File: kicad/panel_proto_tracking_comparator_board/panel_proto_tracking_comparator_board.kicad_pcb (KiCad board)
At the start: 2 copper layers, 60 x 46.4 mm, 384 parts, among them U1 MCP6566

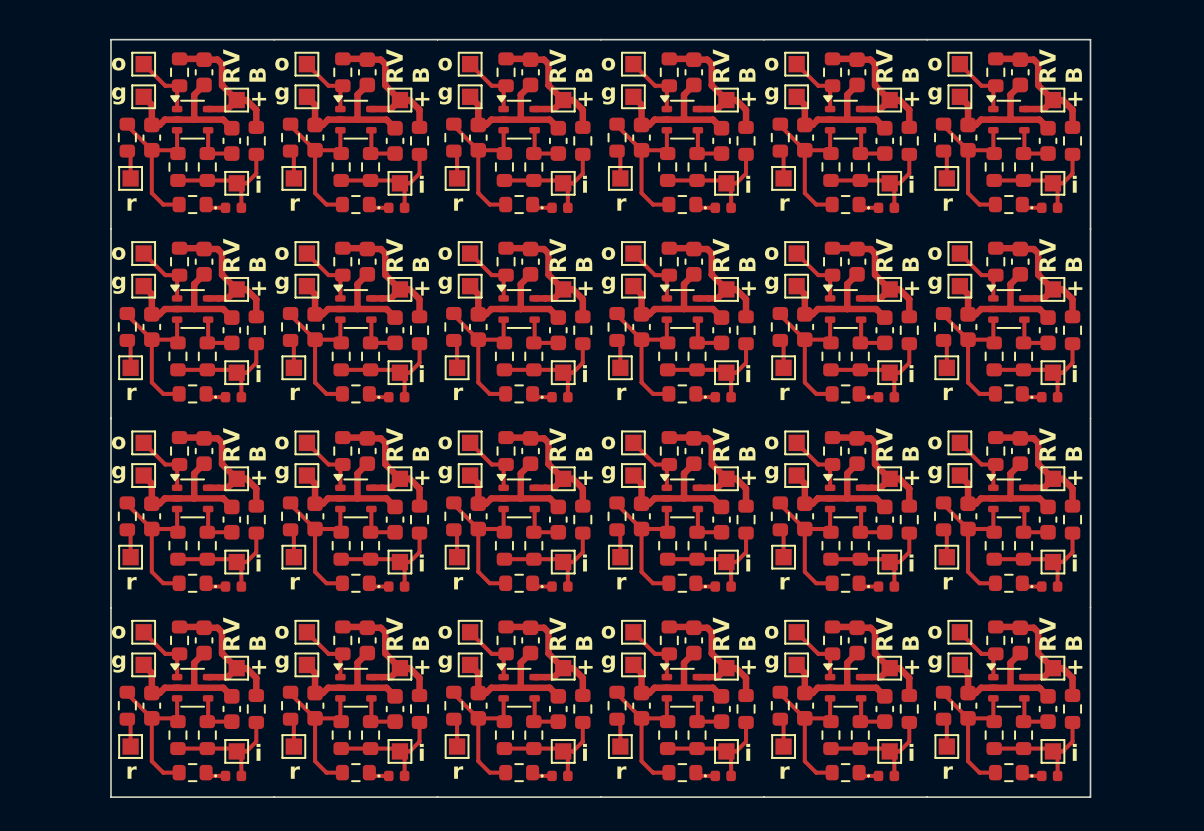
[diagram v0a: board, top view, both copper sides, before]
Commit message: Data slicer rev A
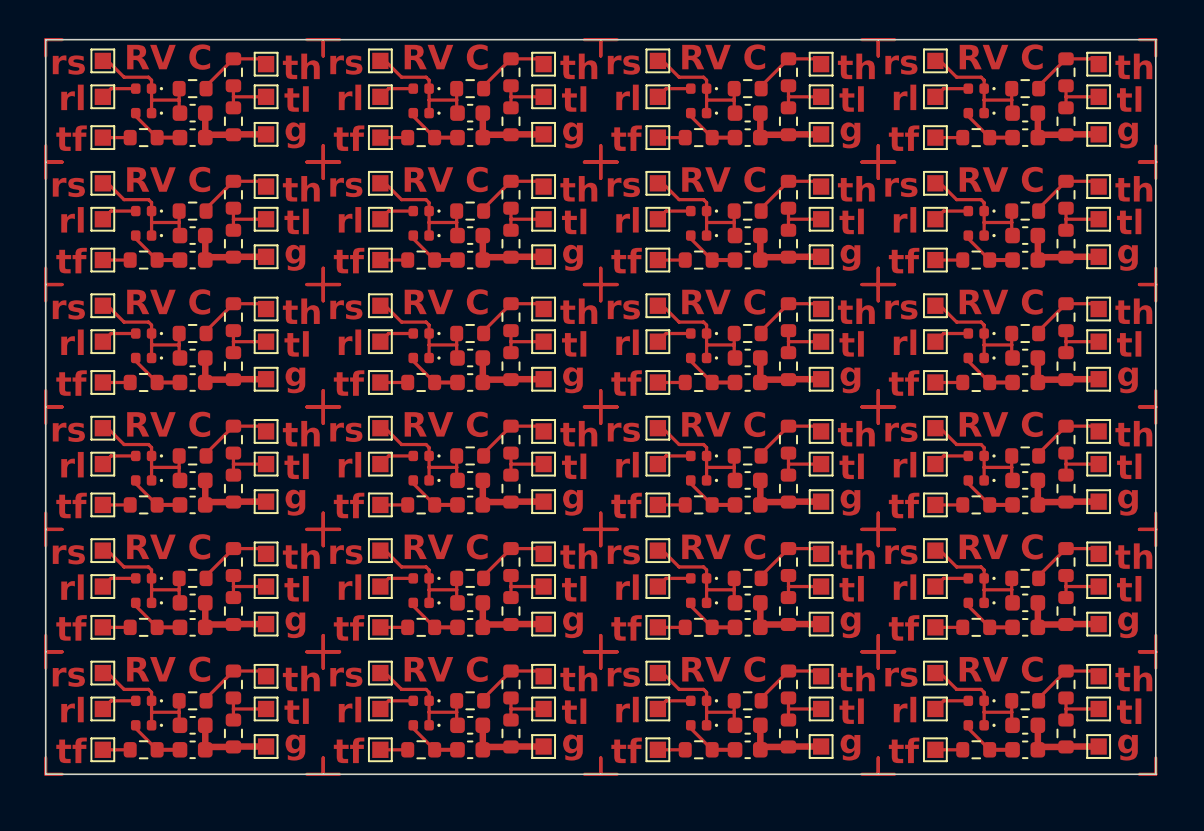
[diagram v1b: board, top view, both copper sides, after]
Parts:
- removed the C1 at (145.4, 33.6)
- removed the C1 at (125.4, 22.0)
- removed the C1 at (135.4, 33.6)
- removed the C1 at (135.4, 56.8)
- removed the C1 at (135.4, 22.0)
- removed the C1 at (135.4, 45.2)
- removed the C1 at (155.4, 33.6)
- removed the C1 at (165.4, 56.8)
- removed the C1 at (115.4, 56.8)
- removed the C1 at (115.4, 45.2)
- removed the C1 at (125.4, 56.8)
- removed the C1 at (155.4, 22.0)
- removed the C1 at (145.4, 22.0)
- removed the C1 at (145.4, 45.2)
- removed the C1 at (155.4, 45.2)
- removed the C1 at (125.4, 33.6)
- removed the C1 at (125.4, 45.2)
- removed the C1 at (165.4, 22.0)
- removed the C1 at (165.4, 33.6)
- removed the C1 at (145.4, 56.8)
- removed the C1 at (155.4, 56.8)
- removed the C1 at (115.4, 22.0)
- removed the C1 at (165.4, 45.2)
- removed the C1 at (115.4, 33.6)
- removed C2 (x24): 100pF, Capacitor_SMD:C_0603_1608Metric
- removed the C3 at (147.1, 49.4)
- removed the C3 at (127.1, 49.4)
- removed the C3 at (157.1, 61.0)
- removed the C3 at (137.1, 26.2)
- removed the C3 at (167.1, 26.2)
- removed the C3 at (157.1, 37.8)
- removed the C3 at (147.1, 61.0)
- removed the C3 at (167.1, 49.4)
- removed the C3 at (127.1, 26.2)
- removed the C3 at (167.1, 37.8)
- removed the C3 at (127.1, 61.0)
- removed the C3 at (137.1, 49.4)
- removed the C3 at (137.1, 61.0)
- removed the C3 at (147.1, 37.8)
- removed the C3 at (117.1, 61.0)
- removed the C3 at (167.1, 61.0)
- removed the C3 at (117.1, 26.2)
- removed the C3 at (127.1, 37.8)
- removed the C3 at (137.1, 37.8)
- removed the C3 at (117.1, 37.8)
- removed the C3 at (157.1, 49.4)
- removed the C3 at (157.1, 26.2)
- removed the C3 at (117.1, 49.4)
- removed the C3 at (147.1, 26.2)
- removed the D1 at (157.2, 30.3)
- removed the D1 at (137.2, 30.3)
- removed the D1 at (137.2, 53.5)
- removed the D1 at (167.2, 30.3)
- removed the D1 at (127.2, 41.9)
- removed the D1 at (127.2, 30.3)
- removed the D1 at (117.2, 41.9)
- removed the D1 at (167.2, 65.1)
- removed the D1 at (117.2, 65.1)
- removed the D1 at (167.2, 41.9)
- removed the D1 at (117.2, 30.3)
- removed the D1 at (117.2, 53.5)
- removed the D1 at (127.2, 65.1)
- removed the D1 at (157.2, 41.9)
- removed the D1 at (147.2, 65.1)
- removed the D1 at (157.2, 53.5)
- removed the D1 at (127.2, 53.5)
- removed the D1 at (157.2, 65.1)
- removed the D1 at (137.2, 65.1)
- removed the D1 at (137.2, 41.9)
- removed the D1 at (147.2, 41.9)
- removed the D1 at (147.2, 53.5)
- removed the D1 at (167.2, 53.5)
- removed the D1 at (147.2, 30.3)
- removed the R1 at (163.8, 51.0)
- removed the R1 at (143.8, 62.6)
- removed the R1 at (143.8, 51.0)
- removed the R1 at (133.8, 39.4)
- removed the R1 at (113.8, 51.0)
- removed the R1 at (133.8, 51.0)
- removed the R1 at (123.8, 51.0)
- removed the R1 at (163.8, 62.6)
- removed the R1 at (153.8, 39.4)
- removed the R1 at (113.8, 39.4)
- removed the R1 at (133.8, 27.8)
- removed the R1 at (123.8, 62.6)
- removed the R1 at (153.8, 51.0)
- removed the R1 at (123.8, 27.8)
- removed the R1 at (153.8, 62.6)
- removed the R1 at (113.8, 27.8)
- removed the R1 at (123.8, 39.4)
- removed the R1 at (143.8, 27.8)
- removed the R1 at (163.8, 27.8)
- removed the R1 at (133.8, 62.6)
- removed the R1 at (163.8, 39.4)
- removed the R1 at (143.8, 39.4)
- removed the R1 at (153.8, 27.8)
- removed the R1 at (113.8, 62.6)
- removed the R2 at (128.6, 26.2)
- removed the R2 at (118.6, 49.4)
- removed the R2 at (158.6, 37.8)
- removed the R2 at (168.6, 49.4)
- removed the R2 at (118.6, 26.2)
- removed the R2 at (118.6, 37.8)
- removed the R2 at (138.6, 61.0)
- removed the R2 at (158.6, 26.2)
- removed the R2 at (168.6, 26.2)
- removed the R2 at (148.6, 49.4)
- removed the R2 at (128.6, 37.8)
- removed the R2 at (168.6, 37.8)
- removed the R2 at (158.6, 49.4)
- removed the R2 at (128.6, 49.4)
- removed the R2 at (148.6, 61.0)
- removed the R2 at (148.6, 37.8)
- removed the R2 at (138.6, 49.4)
- removed the R2 at (128.6, 61.0)
- removed the R2 at (158.6, 61.0)
- removed the R2 at (138.6, 26.2)
- removed the R2 at (148.6, 26.2)
- removed the R2 at (168.6, 61.0)
- removed the R2 at (118.6, 61.0)
- removed the R2 at (138.6, 37.8)
- removed R3 (x24): 1k, Resistor_SMD:R_0603_1608Metric
- removed R4 (x24): 10k, Resistor_SMD:R_0603_1608Metric
- removed the R5 at (135.6, 51.0)
- removed the R5 at (145.6, 62.6)
- removed the R5 at (165.6, 39.4)
- removed the R5 at (155.6, 51.0)
- removed the R5 at (135.6, 39.4)
- removed the R5 at (115.6, 27.8)
- removed the R5 at (155.6, 27.8)
- removed the R5 at (115.6, 51.0)
- removed the R5 at (115.6, 62.6)
- removed the R5 at (115.6, 39.4)
- removed the R5 at (165.6, 51.0)
- removed the R5 at (155.6, 62.6)
- removed the R5 at (145.6, 51.0)
- removed the R5 at (125.6, 51.0)
- removed the R5 at (125.6, 62.6)
- removed the R5 at (135.6, 27.8)
- removed the R5 at (135.6, 62.6)
- removed the R5 at (145.6, 39.4)
- removed the R5 at (125.6, 27.8)
- removed the R5 at (165.6, 62.6)
- removed the R5 at (145.6, 27.8)
- removed the R5 at (165.6, 27.8)
- removed the R5 at (155.6, 39.4)
- removed the R5 at (125.6, 39.4)
- removed R6 (x24): 1M, Resistor_SMD:R_0603_1608Metric
- removed the TP1 at (157.4, 40.4)
- removed the TP1 at (117.4, 63.6)
- removed the TP1 at (137.4, 40.4)
- removed the TP1 at (117.4, 52.0)
- removed the TP1 at (167.4, 52.0)
- removed the TP1 at (147.4, 40.4)
- removed the TP1 at (127.4, 52.0)
- removed the TP1 at (167.4, 40.4)
- removed the TP1 at (147.4, 28.8)
- removed the TP1 at (127.4, 28.8)
- removed the TP1 at (117.4, 40.4)
- removed the TP1 at (127.4, 40.4)
- removed the TP1 at (147.4, 52.0)
- removed the TP1 at (137.4, 28.8)
- removed the TP1 at (117.4, 28.8)
- removed the TP1 at (157.4, 52.0)
- removed the TP1 at (167.4, 63.6)
- removed the TP1 at (167.4, 28.8)
- removed the TP1 at (137.4, 52.0)
- removed the TP1 at (157.4, 63.6)
- removed the TP1 at (157.4, 28.8)
- removed the TP1 at (127.4, 63.6)
- removed the TP1 at (147.4, 63.6)
- removed the TP1 at (137.4, 63.6)
- removed the TP2 at (151.7, 56.3)
- removed the TP2 at (151.7, 33.1)
- removed the TP2 at (121.7, 21.5)
- removed the TP2 at (111.7, 33.1)
- removed the TP2 at (141.7, 44.7)
- removed the TP2 at (131.7, 33.1)
- removed the TP2 at (151.7, 21.5)
- removed the TP2 at (161.7, 33.1)
- removed the TP2 at (141.7, 21.5)
- removed the TP2 at (141.7, 56.3)
- removed the TP2 at (121.7, 44.7)
- removed the TP2 at (151.7, 44.7)
- removed the TP2 at (141.7, 33.1)
- removed the TP2 at (161.7, 44.7)
- removed the TP2 at (131.7, 21.5)
- removed the TP2 at (121.7, 56.3)
- removed the TP2 at (111.7, 44.7)
- removed the TP2 at (121.7, 33.1)
- removed the TP2 at (131.7, 56.3)
- removed the TP2 at (111.7, 21.5)
- removed the TP2 at (161.7, 21.5)
- removed the TP2 at (111.7, 56.3)
- removed the TP2 at (131.7, 44.7)
- removed the TP2 at (161.7, 56.3)
- removed TP3 (x24): TestPoint, TestPoint:TestPoint_Pad_1.0x1.0mm
- removed the TP4 at (161.7, 46.7)
- removed the TP4 at (131.7, 58.3)
- removed the TP4 at (131.7, 46.7)
- removed the TP4 at (161.7, 23.5)
- removed the TP4 at (151.7, 46.7)
- removed the TP4 at (161.7, 35.1)
- removed the TP4 at (131.7, 23.5)
- removed the TP4 at (131.7, 35.1)
- removed the TP4 at (111.7, 58.3)
- removed the TP4 at (141.7, 46.7)
- removed the TP4 at (141.7, 35.1)
- removed the TP4 at (151.7, 58.3)
- removed the TP4 at (111.7, 35.1)
- removed the TP4 at (121.7, 58.3)
- removed the TP4 at (141.7, 58.3)
- removed the TP4 at (121.7, 35.1)
- removed the TP4 at (151.7, 35.1)
- removed the TP4 at (141.7, 23.5)
- removed the TP4 at (161.7, 58.3)
- removed the TP4 at (111.7, 46.7)
- removed the TP4 at (121.7, 23.5)
- removed the TP4 at (151.7, 23.5)
- removed the TP4 at (111.7, 23.5)
- removed the TP4 at (121.7, 46.7)
- removed the TP5 at (140.9, 28.5)
- removed the TP5 at (150.9, 51.7)
- removed the TP5 at (160.9, 40.1)
- removed the TP5 at (120.9, 40.1)
- removed the TP5 at (120.9, 28.5)
- removed the TP5 at (130.9, 63.3)
- removed the TP5 at (140.9, 40.1)
- removed the TP5 at (110.9, 63.3)
- removed the TP5 at (130.9, 51.7)
- removed the TP5 at (110.9, 40.1)
- removed the TP5 at (130.9, 28.5)
- removed the TP5 at (110.9, 51.7)
- removed the TP5 at (140.9, 51.7)
- removed the TP5 at (160.9, 63.3)
- removed the TP5 at (120.9, 51.7)
- removed the TP5 at (160.9, 28.5)
- removed the TP5 at (150.9, 28.5)
- removed the TP5 at (140.9, 63.3)
- removed the TP5 at (120.9, 63.3)
- removed the TP5 at (130.9, 40.1)
- removed the TP5 at (150.9, 63.3)
- removed the TP5 at (160.9, 51.7)
- removed the TP5 at (110.9, 28.5)
- removed the TP5 at (150.9, 40.1)
- removed U1 (x24): MCP6566, Package_TO_SOT_SMD:SOT-353_SC-70-5
- added C1: 0.1uF, Capacitor_SMD:C_0603_1608Metric, F.Cu at (165.7, 41.0)
- added C1: 0.1uF, Capacitor_SMD:C_0603_1608Metric, F.Cu at (114.7, 33.5)
- added C1: 0.1uF, Capacitor_SMD:C_0603_1608Metric, F.Cu at (165.7, 56.0)
- added C1: 0.1uF, Capacitor_SMD:C_0603_1608Metric, F.Cu at (114.7, 41.0)
- added C1: 0.1uF, Capacitor_SMD:C_0603_1608Metric, F.Cu at (114.7, 63.5)
- added C1: 0.1uF, Capacitor_SMD:C_0603_1608Metric, F.Cu at (148.7, 33.5)
- added C1: 0.1uF, Capacitor_SMD:C_0603_1608Metric, F.Cu at (114.7, 56.0)
- added C1: 0.1uF, Capacitor_SMD:C_0603_1608Metric, F.Cu at (131.7, 41.0)
- added C1: 0.1uF, Capacitor_SMD:C_0603_1608Metric, F.Cu at (114.7, 48.5)
- added C1: 0.1uF, Capacitor_SMD:C_0603_1608Metric, F.Cu at (165.7, 26.0)
- added C1: 0.1uF, Capacitor_SMD:C_0603_1608Metric, F.Cu at (165.7, 48.5)
- added C1: 0.1uF, Capacitor_SMD:C_0603_1608Metric, F.Cu at (131.7, 48.5)
- added C1: 0.1uF, Capacitor_SMD:C_0603_1608Metric, F.Cu at (131.7, 33.5)
- added C1: 0.1uF, Capacitor_SMD:C_0603_1608Metric, F.Cu at (148.7, 63.5)
- added C1: 0.1uF, Capacitor_SMD:C_0603_1608Metric, F.Cu at (165.7, 33.5)
- added C1: 0.1uF, Capacitor_SMD:C_0603_1608Metric, F.Cu at (131.7, 63.5)
- added C1: 0.1uF, Capacitor_SMD:C_0603_1608Metric, F.Cu at (131.7, 56.0)
- added C1: 0.1uF, Capacitor_SMD:C_0603_1608Metric, F.Cu at (148.7, 48.5)
- added C1: 0.1uF, Capacitor_SMD:C_0603_1608Metric, F.Cu at (114.7, 26.0)
- added C1: 0.1uF, Capacitor_SMD:C_0603_1608Metric, F.Cu at (148.7, 26.0)
- added C1: 0.1uF, Capacitor_SMD:C_0603_1608Metric, F.Cu at (131.7, 26.0)
- added C1: 0.1uF, Capacitor_SMD:C_0603_1608Metric, F.Cu at (148.7, 56.0)
- added C1: 0.1uF, Capacitor_SMD:C_0603_1608Metric, F.Cu at (165.7, 63.5)
- added C1: 0.1uF, Capacitor_SMD:C_0603_1608Metric, F.Cu at (148.7, 41.0)
- added C3: 1nF, Capacitor_SMD:C_0603_1608Metric, F.Cu at (114.7, 32.0)
- added C3: 1nF, Capacitor_SMD:C_0603_1608Metric, F.Cu at (131.7, 47.0)
- added C3: 1nF, Capacitor_SMD:C_0603_1608Metric, F.Cu at (165.7, 32.0)
- added C3: 1nF, Capacitor_SMD:C_0603_1608Metric, F.Cu at (131.7, 32.0)
- added C3: 1nF, Capacitor_SMD:C_0603_1608Metric, F.Cu at (114.7, 47.0)
- added C3: 1nF, Capacitor_SMD:C_0603_1608Metric, F.Cu at (165.7, 62.0)
- added C3: 1nF, Capacitor_SMD:C_0603_1608Metric, F.Cu at (131.7, 24.5)
- added C3: 1nF, Capacitor_SMD:C_0603_1608Metric, F.Cu at (148.7, 47.0)
- added C3: 1nF, Capacitor_SMD:C_0603_1608Metric, F.Cu at (165.7, 39.5)
- added C3: 1nF, Capacitor_SMD:C_0603_1608Metric, F.Cu at (131.7, 62.0)
- added C3: 1nF, Capacitor_SMD:C_0603_1608Metric, F.Cu at (114.7, 54.5)
- added C3: 1nF, Capacitor_SMD:C_0603_1608Metric, F.Cu at (148.7, 54.5)
- added C3: 1nF, Capacitor_SMD:C_0603_1608Metric, F.Cu at (131.7, 54.5)
- added C3: 1nF, Capacitor_SMD:C_0603_1608Metric, F.Cu at (165.7, 24.5)
- added C3: 1nF, Capacitor_SMD:C_0603_1608Metric, F.Cu at (148.7, 62.0)
- added C3: 1nF, Capacitor_SMD:C_0603_1608Metric, F.Cu at (148.7, 39.5)
- added C3: 1nF, Capacitor_SMD:C_0603_1608Metric, F.Cu at (114.7, 62.0)
- added C3: 1nF, Capacitor_SMD:C_0603_1608Metric, F.Cu at (165.7, 47.0)
- added C3: 1nF, Capacitor_SMD:C_0603_1608Metric, F.Cu at (114.7, 39.5)
- added C3: 1nF, Capacitor_SMD:C_0603_1608Metric, F.Cu at (131.7, 39.5)
- added C3: 1nF, Capacitor_SMD:C_0603_1608Metric, F.Cu at (165.7, 54.5)
- added C3: 1nF, Capacitor_SMD:C_0603_1608Metric, F.Cu at (148.7, 24.5)
- added C3: 1nF, Capacitor_SMD:C_0603_1608Metric, F.Cu at (114.7, 24.5)
- added C3: 1nF, Capacitor_SMD:C_0603_1608Metric, F.Cu at (148.7, 32.0)
- added D1: D_Schottky, Custom_Diode:D_0402_1005Metric, F.Cu at (162.7, 53.0)
- added D1: D_Schottky, Custom_Diode:D_0402_1005Metric, F.Cu at (162.7, 60.5)
- added D1: D_Schottky, Custom_Diode:D_0402_1005Metric, F.Cu at (128.7, 30.5)
- added D1: D_Schottky, Custom_Diode:D_0402_1005Metric, F.Cu at (128.7, 23.0)
- added D1: D_Schottky, Custom_Diode:D_0402_1005Metric, F.Cu at (111.7, 60.5)
- added D1: D_Schottky, Custom_Diode:D_0402_1005Metric, F.Cu at (111.7, 30.5)
- added D1: D_Schottky, Custom_Diode:D_0402_1005Metric, F.Cu at (111.7, 38.0)
- added D1: D_Schottky, Custom_Diode:D_0402_1005Metric, F.Cu at (145.7, 23.0)
- added D1: D_Schottky, Custom_Diode:D_0402_1005Metric, F.Cu at (145.7, 30.5)
- added D1: D_Schottky, Custom_Diode:D_0402_1005Metric, F.Cu at (145.7, 38.0)
- added D1: D_Schottky, Custom_Diode:D_0402_1005Metric, F.Cu at (145.7, 45.5)
- added D1: D_Schottky, Custom_Diode:D_0402_1005Metric, F.Cu at (128.7, 38.0)
- added D1: D_Schottky, Custom_Diode:D_0402_1005Metric, F.Cu at (128.7, 60.5)
- added D1: D_Schottky, Custom_Diode:D_0402_1005Metric, F.Cu at (162.7, 30.5)
- added D1: D_Schottky, Custom_Diode:D_0402_1005Metric, F.Cu at (128.7, 53.0)
- added D1: D_Schottky, Custom_Diode:D_0402_1005Metric, F.Cu at (162.7, 45.5)
- added D1: D_Schottky, Custom_Diode:D_0402_1005Metric, F.Cu at (111.7, 23.0)
- added D1: D_Schottky, Custom_Diode:D_0402_1005Metric, F.Cu at (111.7, 45.5)
- added D1: D_Schottky, Custom_Diode:D_0402_1005Metric, F.Cu at (162.7, 38.0)
- added D1: D_Schottky, Custom_Diode:D_0402_1005Metric, F.Cu at (162.7, 23.0)
- added D1: D_Schottky, Custom_Diode:D_0402_1005Metric, F.Cu at (128.7, 45.5)
- added D1: D_Schottky, Custom_Diode:D_0402_1005Metric, F.Cu at (145.7, 60.5)
- added D1: D_Schottky, Custom_Diode:D_0402_1005Metric, F.Cu at (111.7, 53.0)
- added D1: D_Schottky, Custom_Diode:D_0402_1005Metric, F.Cu at (145.7, 53.0)
- added D2: D_Schottky, Custom_Diode:D_0402_1005Metric, F.Cu at (111.7, 54.5)
- added D2: D_Schottky, Custom_Diode:D_0402_1005Metric, F.Cu at (162.7, 54.5)
- added D2: D_Schottky, Custom_Diode:D_0402_1005Metric, F.Cu at (162.7, 24.5)
- added D2: D_Schottky, Custom_Diode:D_0402_1005Metric, F.Cu at (111.7, 24.5)
- added D2: D_Schottky, Custom_Diode:D_0402_1005Metric, F.Cu at (111.7, 47.0)
- added D2: D_Schottky, Custom_Diode:D_0402_1005Metric, F.Cu at (162.7, 62.0)
- added D2: D_Schottky, Custom_Diode:D_0402_1005Metric, F.Cu at (145.7, 39.5)
- added D2: D_Schottky, Custom_Diode:D_0402_1005Metric, F.Cu at (128.7, 24.5)
- added D2: D_Schottky, Custom_Diode:D_0402_1005Metric, F.Cu at (111.7, 62.0)
- added D2: D_Schottky, Custom_Diode:D_0402_1005Metric, F.Cu at (145.7, 24.5)
- added D2: D_Schottky, Custom_Diode:D_0402_1005Metric, F.Cu at (128.7, 54.5)
- added D2: D_Schottky, Custom_Diode:D_0402_1005Metric, F.Cu at (145.7, 32.0)
- added D2: D_Schottky, Custom_Diode:D_0402_1005Metric, F.Cu at (128.7, 62.0)
- added D2: D_Schottky, Custom_Diode:D_0402_1005Metric, F.Cu at (145.7, 54.5)
- added D2: D_Schottky, Custom_Diode:D_0402_1005Metric, F.Cu at (128.7, 39.5)
- added D2: D_Schottky, Custom_Diode:D_0402_1005Metric, F.Cu at (111.7, 32.0)
- added D2: D_Schottky, Custom_Diode:D_0402_1005Metric, F.Cu at (162.7, 39.5)
- added D2: D_Schottky, Custom_Diode:D_0402_1005Metric, F.Cu at (162.7, 47.0)
- added D2: D_Schottky, Custom_Diode:D_0402_1005Metric, F.Cu at (162.7, 32.0)
- added D2: D_Schottky, Custom_Diode:D_0402_1005Metric, F.Cu at (145.7, 62.0)
- added D2: D_Schottky, Custom_Diode:D_0402_1005Metric, F.Cu at (128.7, 32.0)
- added D2: D_Schottky, Custom_Diode:D_0402_1005Metric, F.Cu at (111.7, 39.5)
- added D2: D_Schottky, Custom_Diode:D_0402_1005Metric, F.Cu at (128.7, 47.0)
- added D2: D_Schottky, Custom_Diode:D_0402_1005Metric, F.Cu at (145.7, 47.0)
- added R1: 10k, Resistor_SMD:R_0603_1608Metric, F.Cu at (111.7, 48.5)
- added R1: 10k, Resistor_SMD:R_0603_1608Metric, F.Cu at (111.7, 56.0)
- added R1: 10k, Resistor_SMD:R_0603_1608Metric, F.Cu at (145.7, 26.0)
- added R1: 10k, Resistor_SMD:R_0603_1608Metric, F.Cu at (162.7, 48.5)
- added R1: 10k, Resistor_SMD:R_0603_1608Metric, F.Cu at (162.7, 56.0)
- added R1: 10k, Resistor_SMD:R_0603_1608Metric, F.Cu at (145.7, 33.5)
- added R1: 10k, Resistor_SMD:R_0603_1608Metric, F.Cu at (162.7, 63.5)
- added R1: 10k, Resistor_SMD:R_0603_1608Metric, F.Cu at (128.7, 26.0)
- added R1: 10k, Resistor_SMD:R_0603_1608Metric, F.Cu at (111.7, 63.5)
- added R1: 10k, Resistor_SMD:R_0603_1608Metric, F.Cu at (162.7, 26.0)
- added R1: 10k, Resistor_SMD:R_0603_1608Metric, F.Cu at (145.7, 63.5)
- added R1: 10k, Resistor_SMD:R_0603_1608Metric, F.Cu at (145.7, 56.0)
- added R1: 10k, Resistor_SMD:R_0603_1608Metric, F.Cu at (162.7, 33.5)
- added R1: 10k, Resistor_SMD:R_0603_1608Metric, F.Cu at (128.7, 33.5)
- added R1: 10k, Resistor_SMD:R_0603_1608Metric, F.Cu at (145.7, 48.5)
- added R1: 10k, Resistor_SMD:R_0603_1608Metric, F.Cu at (111.7, 33.5)
- added R1: 10k, Resistor_SMD:R_0603_1608Metric, F.Cu at (128.7, 41.0)
- added R1: 10k, Resistor_SMD:R_0603_1608Metric, F.Cu at (111.7, 26.0)
- added R1: 10k, Resistor_SMD:R_0603_1608Metric, F.Cu at (128.7, 48.5)
- added R1: 10k, Resistor_SMD:R_0603_1608Metric, F.Cu at (128.7, 56.0)
- added R1: 10k, Resistor_SMD:R_0603_1608Metric, F.Cu at (162.7, 41.0)
- added R1: 10k, Resistor_SMD:R_0603_1608Metric, F.Cu at (128.7, 63.5)
- added R1: 10k, Resistor_SMD:R_0603_1608Metric, F.Cu at (145.7, 41.0)
- added R1: 10k, Resistor_SMD:R_0603_1608Metric, F.Cu at (111.7, 41.0)
- added R2: 100k, Resistor_SMD:R_0603_1608Metric, F.Cu at (134.2, 29.5)
- added R2: 100k, Resistor_SMD:R_0603_1608Metric, F.Cu at (117.2, 29.5)
- added R2: 100k, Resistor_SMD:R_0603_1608Metric, F.Cu at (168.2, 52.0)
- added R2: 100k, Resistor_SMD:R_0603_1608Metric, F.Cu at (134.2, 37.0)
- added R2: 100k, Resistor_SMD:R_0603_1608Metric, F.Cu at (151.2, 59.5)
- added R2: 100k, Resistor_SMD:R_0603_1608Metric, F.Cu at (134.2, 59.5)
- added R2: 100k, Resistor_SMD:R_0603_1608Metric, F.Cu at (168.2, 37.0)
- added R2: 100k, Resistor_SMD:R_0603_1608Metric, F.Cu at (134.2, 44.5)
- added R2: 100k, Resistor_SMD:R_0603_1608Metric, F.Cu at (151.2, 29.5)
- added R2: 100k, Resistor_SMD:R_0603_1608Metric, F.Cu at (151.2, 44.5)
- added R2: 100k, Resistor_SMD:R_0603_1608Metric, F.Cu at (134.2, 22.0)
- added R2: 100k, Resistor_SMD:R_0603_1608Metric, F.Cu at (168.2, 22.0)
- added R2: 100k, Resistor_SMD:R_0603_1608Metric, F.Cu at (117.2, 52.0)
- added R2: 100k, Resistor_SMD:R_0603_1608Metric, F.Cu at (117.2, 59.5)
- added R2: 100k, Resistor_SMD:R_0603_1608Metric, F.Cu at (151.2, 22.0)
- added R2: 100k, Resistor_SMD:R_0603_1608Metric, F.Cu at (117.2, 44.5)
- added R2: 100k, Resistor_SMD:R_0603_1608Metric, F.Cu at (168.2, 44.5)
- added R2: 100k, Resistor_SMD:R_0603_1608Metric, F.Cu at (151.2, 52.0)
- added R2: 100k, Resistor_SMD:R_0603_1608Metric, F.Cu at (117.2, 37.0)
- added R2: 100k, Resistor_SMD:R_0603_1608Metric, F.Cu at (168.2, 59.5)
- added R2: 100k, Resistor_SMD:R_0603_1608Metric, F.Cu at (117.2, 22.0)
- added R2: 100k, Resistor_SMD:R_0603_1608Metric, F.Cu at (151.2, 37.0)
- added R2: 100k, Resistor_SMD:R_0603_1608Metric, F.Cu at (168.2, 29.5)
- added R2: 100k, Resistor_SMD:R_0603_1608Metric, F.Cu at (134.2, 52.0)
- added R5: 100k, Resistor_SMD:R_0603_1608Metric, F.Cu at (165.7, 45.5)
- added R5: 100k, Resistor_SMD:R_0603_1608Metric, F.Cu at (114.7, 23.0)
- added R5: 100k, Resistor_SMD:R_0603_1608Metric, F.Cu at (131.7, 23.0)
- added R5: 100k, Resistor_SMD:R_0603_1608Metric, F.Cu at (148.7, 23.0)
- added R5: 100k, Resistor_SMD:R_0603_1608Metric, F.Cu at (131.7, 30.5)
- added R5: 100k, Resistor_SMD:R_0603_1608Metric, F.Cu at (114.7, 30.5)
- added R5: 100k, Resistor_SMD:R_0603_1608Metric, F.Cu at (165.7, 23.0)
- added R5: 100k, Resistor_SMD:R_0603_1608Metric, F.Cu at (131.7, 60.5)
- added R5: 100k, Resistor_SMD:R_0603_1608Metric, F.Cu at (148.7, 30.5)
- added R5: 100k, Resistor_SMD:R_0603_1608Metric, F.Cu at (131.7, 53.0)
- added R5: 100k, Resistor_SMD:R_0603_1608Metric, F.Cu at (165.7, 60.5)
- added R5: 100k, Resistor_SMD:R_0603_1608Metric, F.Cu at (148.7, 53.0)
- added R5: 100k, Resistor_SMD:R_0603_1608Metric, F.Cu at (131.7, 45.5)
- added R5: 100k, Resistor_SMD:R_0603_1608Metric, F.Cu at (131.7, 38.0)
- added R5: 100k, Resistor_SMD:R_0603_1608Metric, F.Cu at (148.7, 60.5)
- added R5: 100k, Resistor_SMD:R_0603_1608Metric, F.Cu at (165.7, 38.0)
- added R5: 100k, Resistor_SMD:R_0603_1608Metric, F.Cu at (148.7, 38.0)
- added R5: 100k, Resistor_SMD:R_0603_1608Metric, F.Cu at (165.7, 30.5)
- added R5: 100k, Resistor_SMD:R_0603_1608Metric, F.Cu at (114.7, 53.0)
- added R5: 100k, Resistor_SMD:R_0603_1608Metric, F.Cu at (114.7, 38.0)
- added R5: 100k, Resistor_SMD:R_0603_1608Metric, F.Cu at (148.7, 45.5)
- added R5: 100k, Resistor_SMD:R_0603_1608Metric, F.Cu at (114.7, 45.5)
- added R5: 100k, Resistor_SMD:R_0603_1608Metric, F.Cu at (114.7, 60.5)
- added R5: 100k, Resistor_SMD:R_0603_1608Metric, F.Cu at (165.7, 53.0)
- added R7: 200k, Resistor_SMD:R_0603_1608Metric, F.Cu at (134.2, 32.5)
- added R7: 200k, Resistor_SMD:R_0603_1608Metric, F.Cu at (117.2, 25.0)
- added R7: 200k, Resistor_SMD:R_0603_1608Metric, F.Cu at (117.2, 32.5)
- added R7: 200k, Resistor_SMD:R_0603_1608Metric, F.Cu at (151.2, 47.5)
- added R7: 200k, Resistor_SMD:R_0603_1608Metric, F.Cu at (117.2, 62.5)
- added R7: 200k, Resistor_SMD:R_0603_1608Metric, F.Cu at (168.2, 55.0)
- added R7: 200k, Resistor_SMD:R_0603_1608Metric, F.Cu at (168.2, 25.0)
- added R7: 200k, Resistor_SMD:R_0603_1608Metric, F.Cu at (151.2, 32.5)
- added R7: 200k, Resistor_SMD:R_0603_1608Metric, F.Cu at (134.2, 40.0)
- added R7: 200k, Resistor_SMD:R_0603_1608Metric, F.Cu at (117.2, 40.0)
- added R7: 200k, Resistor_SMD:R_0603_1608Metric, F.Cu at (151.2, 62.5)
- added R7: 200k, Resistor_SMD:R_0603_1608Metric, F.Cu at (168.2, 32.5)
- added R7: 200k, Resistor_SMD:R_0603_1608Metric, F.Cu at (134.2, 25.0)
- added R7: 200k, Resistor_SMD:R_0603_1608Metric, F.Cu at (134.2, 62.5)
- added R7: 200k, Resistor_SMD:R_0603_1608Metric, F.Cu at (168.2, 62.5)
- added R7: 200k, Resistor_SMD:R_0603_1608Metric, F.Cu at (168.2, 40.0)
- added R7: 200k, Resistor_SMD:R_0603_1608Metric, F.Cu at (134.2, 55.0)
- added R7: 200k, Resistor_SMD:R_0603_1608Metric, F.Cu at (151.2, 55.0)
- added R7: 200k, Resistor_SMD:R_0603_1608Metric, F.Cu at (151.2, 25.0)
- added R7: 200k, Resistor_SMD:R_0603_1608Metric, F.Cu at (134.2, 47.5)
- added R7: 200k, Resistor_SMD:R_0603_1608Metric, F.Cu at (151.2, 40.0)
- added R7: 200k, Resistor_SMD:R_0603_1608Metric, F.Cu at (117.2, 55.0)
- added R7: 200k, Resistor_SMD:R_0603_1608Metric, F.Cu at (168.2, 47.5)
- added R7: 200k, Resistor_SMD:R_0603_1608Metric, F.Cu at (117.2, 47.5)
- added TP1: TestPoint, TestPoint:TestPoint_Pad_1.0x1.0mm, F.Cu at (109.2, 31.0)
- added TP1: TestPoint, TestPoint:TestPoint_Pad_1.0x1.0mm, F.Cu at (126.2, 38.5)
- added TP1: TestPoint, TestPoint:TestPoint_Pad_1.0x1.0mm, F.Cu at (143.2, 46.0)
- added TP1: TestPoint, TestPoint:TestPoint_Pad_1.0x1.0mm, F.Cu at (143.2, 23.5)
- added TP1: TestPoint, TestPoint:TestPoint_Pad_1.0x1.0mm, F.Cu at (160.2, 61.0)
- added TP1: TestPoint, TestPoint:TestPoint_Pad_1.0x1.0mm, F.Cu at (143.2, 31.0)
- added TP1: TestPoint, TestPoint:TestPoint_Pad_1.0x1.0mm, F.Cu at (160.2, 31.0)
- added TP1: TestPoint, TestPoint:TestPoint_Pad_1.0x1.0mm, F.Cu at (109.2, 38.5)
- added TP1: TestPoint, TestPoint:TestPoint_Pad_1.0x1.0mm, F.Cu at (109.2, 53.5)
- added TP1: TestPoint, TestPoint:TestPoint_Pad_1.0x1.0mm, F.Cu at (126.2, 46.0)
- added TP1: TestPoint, TestPoint:TestPoint_Pad_1.0x1.0mm, F.Cu at (160.2, 53.5)
- added TP1: TestPoint, TestPoint:TestPoint_Pad_1.0x1.0mm, F.Cu at (126.2, 53.5)
- added TP1: TestPoint, TestPoint:TestPoint_Pad_1.0x1.0mm, F.Cu at (126.2, 31.0)
- added TP1: TestPoint, TestPoint:TestPoint_Pad_1.0x1.0mm, F.Cu at (160.2, 38.5)
- added TP1: TestPoint, TestPoint:TestPoint_Pad_1.0x1.0mm, F.Cu at (160.2, 23.5)
- added TP1: TestPoint, TestPoint:TestPoint_Pad_1.0x1.0mm, F.Cu at (126.2, 23.5)
- added TP1: TestPoint, TestPoint:TestPoint_Pad_1.0x1.0mm, F.Cu at (109.2, 23.5)
- added TP1: TestPoint, TestPoint:TestPoint_Pad_1.0x1.0mm, F.Cu at (143.2, 38.5)
- added TP1: TestPoint, TestPoint:TestPoint_Pad_1.0x1.0mm, F.Cu at (160.2, 46.0)
- added TP1: TestPoint, TestPoint:TestPoint_Pad_1.0x1.0mm, F.Cu at (143.2, 61.0)
- added TP1: TestPoint, TestPoint:TestPoint_Pad_1.0x1.0mm, F.Cu at (109.2, 46.0)
- added TP1: TestPoint, TestPoint:TestPoint_Pad_1.0x1.0mm, F.Cu at (109.2, 61.0)
- added TP1: TestPoint, TestPoint:TestPoint_Pad_1.0x1.0mm, F.Cu at (143.2, 53.5)
- added TP1: TestPoint, TestPoint:TestPoint_Pad_1.0x1.0mm, F.Cu at (126.2, 61.0)
- added TP2: TestPoint, TestPoint:TestPoint_Pad_1.0x1.0mm, F.Cu at (109.2, 41.0)
- added TP2: TestPoint, TestPoint:TestPoint_Pad_1.0x1.0mm, F.Cu at (126.2, 26.0)
- added TP2: TestPoint, TestPoint:TestPoint_Pad_1.0x1.0mm, F.Cu at (160.2, 41.0)
- added TP2: TestPoint, TestPoint:TestPoint_Pad_1.0x1.0mm, F.Cu at (143.2, 63.5)
- added TP2: TestPoint, TestPoint:TestPoint_Pad_1.0x1.0mm, F.Cu at (109.2, 33.5)
- added TP2: TestPoint, TestPoint:TestPoint_Pad_1.0x1.0mm, F.Cu at (160.2, 33.5)
- added TP2: TestPoint, TestPoint:TestPoint_Pad_1.0x1.0mm, F.Cu at (160.2, 48.5)
- added TP2: TestPoint, TestPoint:TestPoint_Pad_1.0x1.0mm, F.Cu at (109.2, 63.5)
- added TP2: TestPoint, TestPoint:TestPoint_Pad_1.0x1.0mm, F.Cu at (160.2, 56.0)
- added TP2: TestPoint, TestPoint:TestPoint_Pad_1.0x1.0mm, F.Cu at (160.2, 26.0)
- added TP2: TestPoint, TestPoint:TestPoint_Pad_1.0x1.0mm, F.Cu at (143.2, 56.0)
- added TP2: TestPoint, TestPoint:TestPoint_Pad_1.0x1.0mm, F.Cu at (126.2, 56.0)
- added TP2: TestPoint, TestPoint:TestPoint_Pad_1.0x1.0mm, F.Cu at (143.2, 26.0)
- added TP2: TestPoint, TestPoint:TestPoint_Pad_1.0x1.0mm, F.Cu at (143.2, 33.5)
- added TP2: TestPoint, TestPoint:TestPoint_Pad_1.0x1.0mm, F.Cu at (143.2, 48.5)
- added TP2: TestPoint, TestPoint:TestPoint_Pad_1.0x1.0mm, F.Cu at (143.2, 41.0)
- added TP2: TestPoint, TestPoint:TestPoint_Pad_1.0x1.0mm, F.Cu at (160.2, 63.5)
- added TP2: TestPoint, TestPoint:TestPoint_Pad_1.0x1.0mm, F.Cu at (126.2, 48.5)
- added TP2: TestPoint, TestPoint:TestPoint_Pad_1.0x1.0mm, F.Cu at (126.2, 63.5)
- added TP2: TestPoint, TestPoint:TestPoint_Pad_1.0x1.0mm, F.Cu at (126.2, 41.0)
- added TP2: TestPoint, TestPoint:TestPoint_Pad_1.0x1.0mm, F.Cu at (109.2, 48.5)
- added TP2: TestPoint, TestPoint:TestPoint_Pad_1.0x1.0mm, F.Cu at (109.2, 56.0)
- added TP2: TestPoint, TestPoint:TestPoint_Pad_1.0x1.0mm, F.Cu at (126.2, 33.5)
- added TP2: TestPoint, TestPoint:TestPoint_Pad_1.0x1.0mm, F.Cu at (109.2, 26.0)
- added TP4: TestPoint, TestPoint:TestPoint_Pad_1.0x1.0mm, F.Cu at (153.2, 55.8)
- added TP4: TestPoint, TestPoint:TestPoint_Pad_1.0x1.0mm, F.Cu at (119.2, 25.8)
- added TP4: TestPoint, TestPoint:TestPoint_Pad_1.0x1.0mm, F.Cu at (153.2, 25.8)
- added TP4: TestPoint, TestPoint:TestPoint_Pad_1.0x1.0mm, F.Cu at (119.2, 33.3)
- added TP4: TestPoint, TestPoint:TestPoint_Pad_1.0x1.0mm, F.Cu at (136.2, 25.8)
- added TP4: TestPoint, TestPoint:TestPoint_Pad_1.0x1.0mm, F.Cu at (136.2, 63.3)
- added TP4: TestPoint, TestPoint:TestPoint_Pad_1.0x1.0mm, F.Cu at (153.2, 40.8)
- added TP4: TestPoint, TestPoint:TestPoint_Pad_1.0x1.0mm, F.Cu at (170.2, 25.8)
- added TP4: TestPoint, TestPoint:TestPoint_Pad_1.0x1.0mm, F.Cu at (170.2, 48.3)
- added TP4: TestPoint, TestPoint:TestPoint_Pad_1.0x1.0mm, F.Cu at (170.2, 63.3)
- added TP4: TestPoint, TestPoint:TestPoint_Pad_1.0x1.0mm, F.Cu at (119.2, 48.3)
- added TP4: TestPoint, TestPoint:TestPoint_Pad_1.0x1.0mm, F.Cu at (170.2, 33.3)
- added TP4: TestPoint, TestPoint:TestPoint_Pad_1.0x1.0mm, F.Cu at (119.2, 55.8)
- added TP4: TestPoint, TestPoint:TestPoint_Pad_1.0x1.0mm, F.Cu at (136.2, 48.3)
- added TP4: TestPoint, TestPoint:TestPoint_Pad_1.0x1.0mm, F.Cu at (119.2, 63.3)
- added TP4: TestPoint, TestPoint:TestPoint_Pad_1.0x1.0mm, F.Cu at (119.2, 40.8)
- added TP4: TestPoint, TestPoint:TestPoint_Pad_1.0x1.0mm, F.Cu at (153.2, 63.3)
- added TP4: TestPoint, TestPoint:TestPoint_Pad_1.0x1.0mm, F.Cu at (136.2, 55.8)
- added TP4: TestPoint, TestPoint:TestPoint_Pad_1.0x1.0mm, F.Cu at (153.2, 48.3)
- added TP4: TestPoint, TestPoint:TestPoint_Pad_1.0x1.0mm, F.Cu at (136.2, 40.8)
- added TP4: TestPoint, TestPoint:TestPoint_Pad_1.0x1.0mm, F.Cu at (170.2, 55.8)
- added TP4: TestPoint, TestPoint:TestPoint_Pad_1.0x1.0mm, F.Cu at (170.2, 40.8)
- added TP4: TestPoint, TestPoint:TestPoint_Pad_1.0x1.0mm, F.Cu at (153.2, 33.3)
- added TP4: TestPoint, TestPoint:TestPoint_Pad_1.0x1.0mm, F.Cu at (136.2, 33.3)
- added TP5: TestPoint, TestPoint:TestPoint_Pad_1.0x1.0mm, F.Cu at (126.2, 43.8)
- added TP5: TestPoint, TestPoint:TestPoint_Pad_1.0x1.0mm, F.Cu at (143.2, 28.8)
- added TP5: TestPoint, TestPoint:TestPoint_Pad_1.0x1.0mm, F.Cu at (109.2, 21.3)
- added TP5: TestPoint, TestPoint:TestPoint_Pad_1.0x1.0mm, F.Cu at (109.2, 51.3)
- added TP5: TestPoint, TestPoint:TestPoint_Pad_1.0x1.0mm, F.Cu at (143.2, 51.3)
- added TP5: TestPoint, TestPoint:TestPoint_Pad_1.0x1.0mm, F.Cu at (126.2, 28.8)
- added TP5: TestPoint, TestPoint:TestPoint_Pad_1.0x1.0mm, F.Cu at (160.2, 43.8)
- added TP5: TestPoint, TestPoint:TestPoint_Pad_1.0x1.0mm, F.Cu at (109.2, 43.8)
- added TP5: TestPoint, TestPoint:TestPoint_Pad_1.0x1.0mm, F.Cu at (126.2, 58.8)
- added TP5: TestPoint, TestPoint:TestPoint_Pad_1.0x1.0mm, F.Cu at (109.2, 36.3)
- added TP5: TestPoint, TestPoint:TestPoint_Pad_1.0x1.0mm, F.Cu at (160.2, 36.3)
- added TP5: TestPoint, TestPoint:TestPoint_Pad_1.0x1.0mm, F.Cu at (160.2, 58.8)
- added TP5: TestPoint, TestPoint:TestPoint_Pad_1.0x1.0mm, F.Cu at (143.2, 21.3)
- added TP5: TestPoint, TestPoint:TestPoint_Pad_1.0x1.0mm, F.Cu at (160.2, 21.3)
- added TP5: TestPoint, TestPoint:TestPoint_Pad_1.0x1.0mm, F.Cu at (160.2, 51.3)
- added TP5: TestPoint, TestPoint:TestPoint_Pad_1.0x1.0mm, F.Cu at (143.2, 58.8)
- added TP5: TestPoint, TestPoint:TestPoint_Pad_1.0x1.0mm, F.Cu at (109.2, 58.8)
- added TP5: TestPoint, TestPoint:TestPoint_Pad_1.0x1.0mm, F.Cu at (160.2, 28.8)
- added TP5: TestPoint, TestPoint:TestPoint_Pad_1.0x1.0mm, F.Cu at (143.2, 43.8)
- added TP5: TestPoint, TestPoint:TestPoint_Pad_1.0x1.0mm, F.Cu at (143.2, 36.3)
- added TP5: TestPoint, TestPoint:TestPoint_Pad_1.0x1.0mm, F.Cu at (109.2, 28.8)
- added TP5: TestPoint, TestPoint:TestPoint_Pad_1.0x1.0mm, F.Cu at (126.2, 36.3)
- added TP5: TestPoint, TestPoint:TestPoint_Pad_1.0x1.0mm, F.Cu at (126.2, 21.3)
- added TP5: TestPoint, TestPoint:TestPoint_Pad_1.0x1.0mm, F.Cu at (126.2, 51.3)
- added TP6: TestPoint, TestPoint:TestPoint_Pad_1.0x1.0mm, F.Cu at (170.2, 36.5)
- added TP6: TestPoint, TestPoint:TestPoint_Pad_1.0x1.0mm, F.Cu at (153.2, 21.5)
- added TP6: TestPoint, TestPoint:TestPoint_Pad_1.0x1.0mm, F.Cu at (170.2, 29.0)
- added TP6: TestPoint, TestPoint:TestPoint_Pad_1.0x1.0mm, F.Cu at (153.2, 44.0)
- added TP6: TestPoint, TestPoint:TestPoint_Pad_1.0x1.0mm, F.Cu at (119.2, 21.5)
- added TP6: TestPoint, TestPoint:TestPoint_Pad_1.0x1.0mm, F.Cu at (153.2, 59.0)
- added TP6: TestPoint, TestPoint:TestPoint_Pad_1.0x1.0mm, F.Cu at (170.2, 51.5)
- added TP6: TestPoint, TestPoint:TestPoint_Pad_1.0x1.0mm, F.Cu at (136.2, 29.0)
- added TP6: TestPoint, TestPoint:TestPoint_Pad_1.0x1.0mm, F.Cu at (119.2, 29.0)
- added TP6: TestPoint, TestPoint:TestPoint_Pad_1.0x1.0mm, F.Cu at (153.2, 36.5)
- added TP6: TestPoint, TestPoint:TestPoint_Pad_1.0x1.0mm, F.Cu at (119.2, 36.5)
- added TP6: TestPoint, TestPoint:TestPoint_Pad_1.0x1.0mm, F.Cu at (136.2, 36.5)
- added TP6: TestPoint, TestPoint:TestPoint_Pad_1.0x1.0mm, F.Cu at (136.2, 44.0)
- added TP6: TestPoint, TestPoint:TestPoint_Pad_1.0x1.0mm, F.Cu at (136.2, 51.5)
- added TP6: TestPoint, TestPoint:TestPoint_Pad_1.0x1.0mm, F.Cu at (153.2, 51.5)
- added TP6: TestPoint, TestPoint:TestPoint_Pad_1.0x1.0mm, F.Cu at (119.2, 59.0)
- added TP6: TestPoint, TestPoint:TestPoint_Pad_1.0x1.0mm, F.Cu at (170.2, 44.0)
- added TP6: TestPoint, TestPoint:TestPoint_Pad_1.0x1.0mm, F.Cu at (136.2, 21.5)
- added TP6: TestPoint, TestPoint:TestPoint_Pad_1.0x1.0mm, F.Cu at (119.2, 51.5)
- added TP6: TestPoint, TestPoint:TestPoint_Pad_1.0x1.0mm, F.Cu at (153.2, 29.0)
- added TP6: TestPoint, TestPoint:TestPoint_Pad_1.0x1.0mm, F.Cu at (170.2, 21.5)
- added TP6: TestPoint, TestPoint:TestPoint_Pad_1.0x1.0mm, F.Cu at (136.2, 59.0)
- added TP6: TestPoint, TestPoint:TestPoint_Pad_1.0x1.0mm, F.Cu at (119.2, 44.0)
- added TP6: TestPoint, TestPoint:TestPoint_Pad_1.0x1.0mm, F.Cu at (170.2, 59.0)
- added TP7: TestPoint, TestPoint:TestPoint_Pad_1.0x1.0mm, F.Cu at (153.2, 61.0)
- added TP7: TestPoint, TestPoint:TestPoint_Pad_1.0x1.0mm, F.Cu at (119.2, 31.0)
- added TP7: TestPoint, TestPoint:TestPoint_Pad_1.0x1.0mm, F.Cu at (119.2, 53.5)
- added TP7: TestPoint, TestPoint:TestPoint_Pad_1.0x1.0mm, F.Cu at (136.2, 53.5)
- added TP7: TestPoint, TestPoint:TestPoint_Pad_1.0x1.0mm, F.Cu at (153.2, 23.5)
- added TP7: TestPoint, TestPoint:TestPoint_Pad_1.0x1.0mm, F.Cu at (170.2, 46.0)
- added TP7: TestPoint, TestPoint:TestPoint_Pad_1.0x1.0mm, F.Cu at (136.2, 31.0)
- added TP7: TestPoint, TestPoint:TestPoint_Pad_1.0x1.0mm, F.Cu at (153.2, 53.5)
- added TP7: TestPoint, TestPoint:TestPoint_Pad_1.0x1.0mm, F.Cu at (119.2, 61.0)
- added TP7: TestPoint, TestPoint:TestPoint_Pad_1.0x1.0mm, F.Cu at (136.2, 46.0)
- added TP7: TestPoint, TestPoint:TestPoint_Pad_1.0x1.0mm, F.Cu at (119.2, 46.0)
- added TP7: TestPoint, TestPoint:TestPoint_Pad_1.0x1.0mm, F.Cu at (153.2, 31.0)
- added TP7: TestPoint, TestPoint:TestPoint_Pad_1.0x1.0mm, F.Cu at (153.2, 46.0)
- added TP7: TestPoint, TestPoint:TestPoint_Pad_1.0x1.0mm, F.Cu at (170.2, 53.5)
- added TP7: TestPoint, TestPoint:TestPoint_Pad_1.0x1.0mm, F.Cu at (170.2, 38.5)
- added TP7: TestPoint, TestPoint:TestPoint_Pad_1.0x1.0mm, F.Cu at (119.2, 23.5)
- added TP7: TestPoint, TestPoint:TestPoint_Pad_1.0x1.0mm, F.Cu at (170.2, 23.5)
- added TP7: TestPoint, TestPoint:TestPoint_Pad_1.0x1.0mm, F.Cu at (136.2, 38.5)
- added TP7: TestPoint, TestPoint:TestPoint_Pad_1.0x1.0mm, F.Cu at (170.2, 61.0)
- added TP7: TestPoint, TestPoint:TestPoint_Pad_1.0x1.0mm, F.Cu at (136.2, 61.0)
- added TP7: TestPoint, TestPoint:TestPoint_Pad_1.0x1.0mm, F.Cu at (153.2, 38.5)
- added TP7: TestPoint, TestPoint:TestPoint_Pad_1.0x1.0mm, F.Cu at (136.2, 23.5)
- added TP7: TestPoint, TestPoint:TestPoint_Pad_1.0x1.0mm, F.Cu at (170.2, 31.0)
- added TP7: TestPoint, TestPoint:TestPoint_Pad_1.0x1.0mm, F.Cu at (119.2, 38.5)
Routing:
- net Board_9-Net-(U1-+): track 9.94 -> 0.00 mm
- net Board_8-Net-(U1-+): track 9.94 -> 0.00 mm
- net Board_10-Net-(U1-+): track 9.94 -> 0.00 mm
- net Board_11-Net-(U1-+): track 9.94 -> 0.00 mm
- net Board_3-Net-(U1-+): track 9.94 -> 0.00 mm
- net Board_5-Net-(U1-+): track 9.94 -> 0.00 mm
- net Board_4-Net-(U1-+): track 9.94 -> 0.00 mm
- net Board_2-Net-(U1-+): track 9.94 -> 0.00 mm
- net Board_23-Net-(U1-+): track 9.94 -> 0.00 mm
- net Board_22-Net-(U1-+): track 9.94 -> 0.00 mm
- net Board_21-Net-(U1-+): track 9.94 -> 0.00 mm
- net Board_20-Net-(U1-+): track 9.94 -> 0.00 mm
- net Board_17-Net-(U1-+): track 9.94 -> 0.00 mm
- net Board_14-Net-(U1-+): track 9.94 -> 0.00 mm
- net Board_16-Net-(U1-+): track 9.94 -> 0.00 mm
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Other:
- board size 60 x 46.4 mm -> 68 x 45 mm
- board text added: "RV C"
- board text added: "rl"
- board text added: "rs"
- board text added: "tf"
- board text added: "th"
- board text added: "tl"
- board text removed: "+"
- board text removed: "RV B"
- board text removed: "V-CUT"
- board text removed: "i"
- board text removed: "o"
- board text removed: "r"
